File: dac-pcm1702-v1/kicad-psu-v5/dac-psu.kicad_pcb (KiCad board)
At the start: 2 copper layers, 123.2 x 81.3 mm, 81 parts, among them J1 AC, J10 LED, J11 GND, J12 +5V, J13 GND, J14 EARTH, J15 +17V, J16 -17V, J2 GND, J3 AC, J4 +15V, J5 GND, J6 -15V, J7 +5V, J8 GND, J9 -5V, U1 LM317_TO-220, U2 LT3045xMSE, U3 LT3094xMSE, U4 LT3045xMSE, U5 LT3094xMSE, U6 LM317_TO-220, U7 LM337_TO220

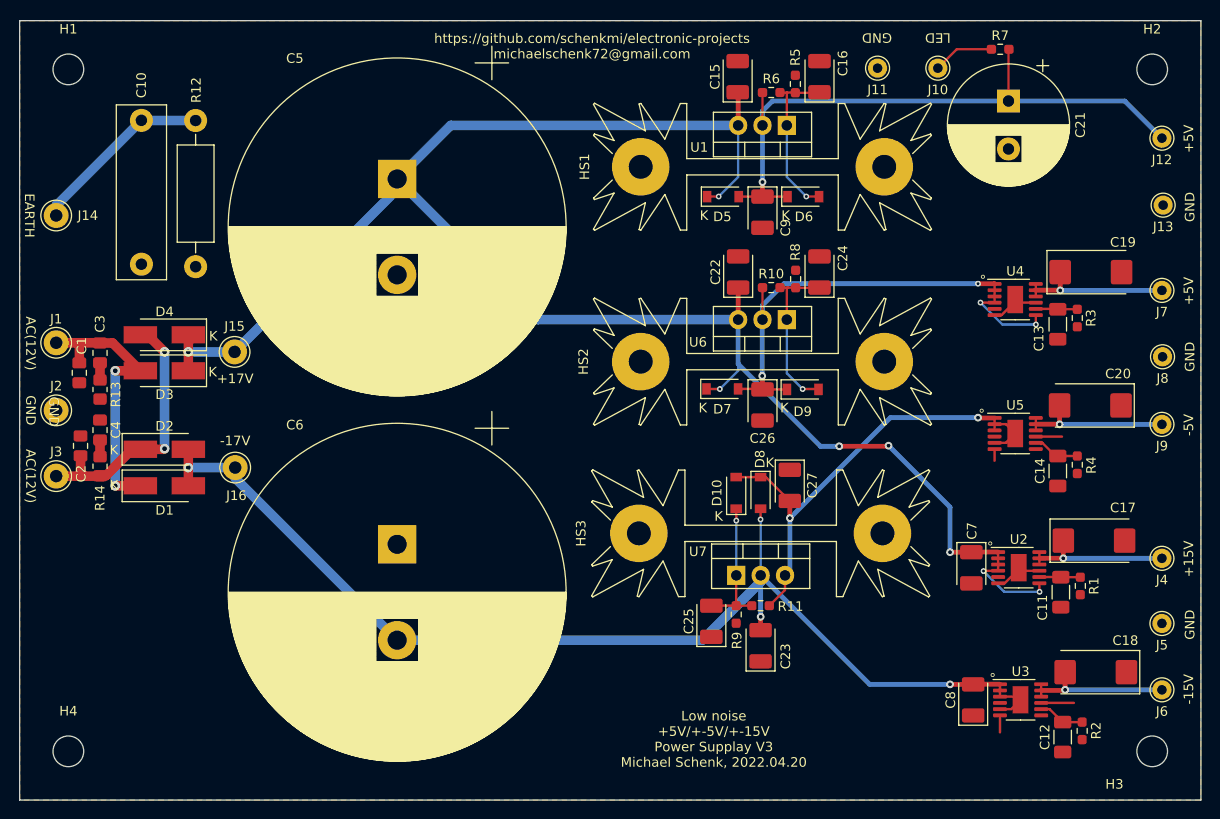
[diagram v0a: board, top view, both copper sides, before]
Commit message: Finalize V5 PSU
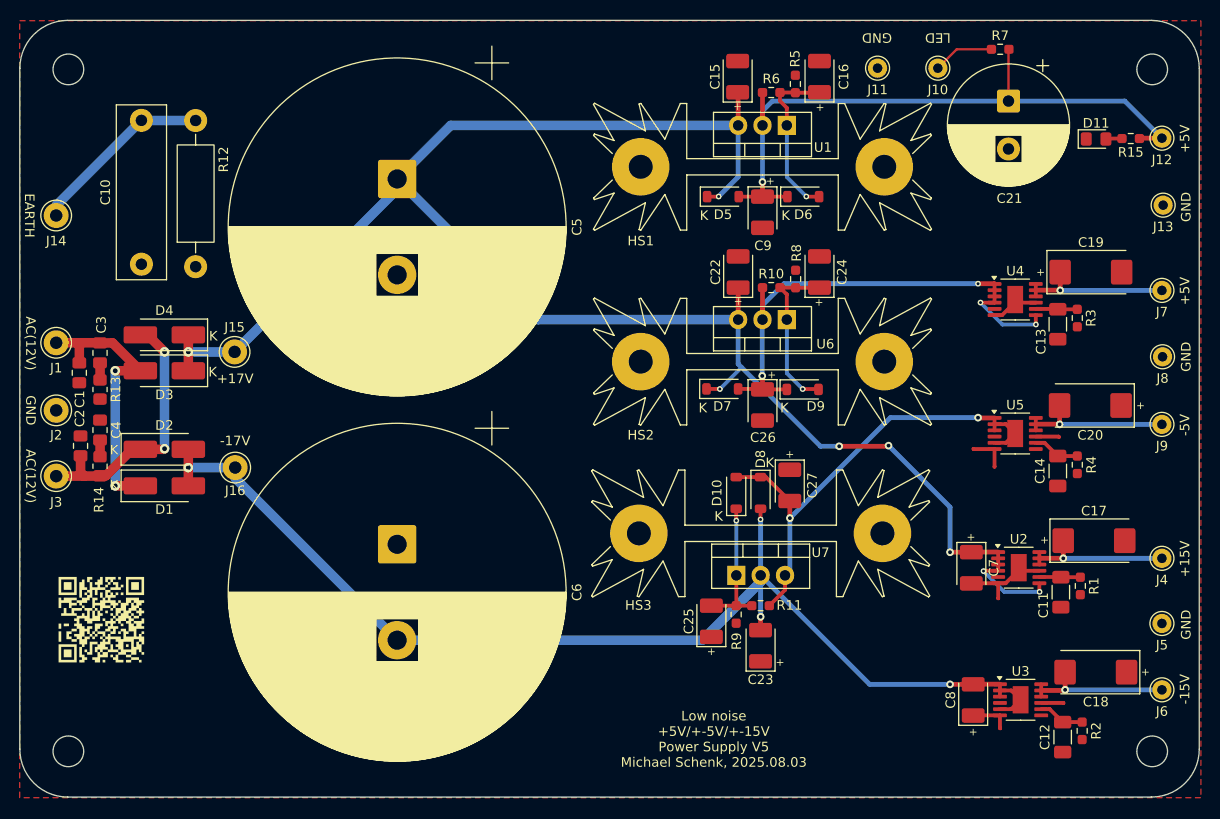
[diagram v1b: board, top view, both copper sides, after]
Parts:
- added D11: LED, LED_SMD:LED_0805_2012Metric_Pad1.15x1.40mm_HandSolder, F.Cu at (206.2, 61.9)
- added G***: LOGO, LOGO, F.Cu at (102.5, 112.0)
- added R15: 330R, Resistor_SMD:R_0603_1608Metric_Pad0.98x0.95mm_HandSolder, F.Cu at (209.9, 61.8)
- C15, C16, C22, C23, C24, C25, C26, C27, C7, C8, C9: footprint Capacitor_Tantalum_SMD:CP_EIA-3528-21_Kemet-B_Pad1.50x2.35mm_HandSolder -> Capacitor_Tantalum_SMD:CP_EIA-3528-21_Kemet-B_HandSolder
- C17, C18, C19, C20: value 47uF -> 47uF/25V; footprint Capacitor_Tantalum_SMD:CP_EIA-7343-31_Kemet-D_Pad2.25x2.55mm_HandSolder -> Capacitor_Tantalum_SMD:CP_EIA-7343-31_Kemet-D_HandSolder
- U2, U3, U4, U5: footprint Package_SO:MSOP-12-1EP_3x4mm_P0.65mm_EP1.65x2.85mm -> Package_SO:MSOP-12-1EP_3x4.039mm_P0.65mm_EP1.651x2.845mm
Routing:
- net GND: track 18.3 -> 28.0 mm
- net +17V: track 191.4 -> 186.7 mm
- net Net-(D5-A): track 66.5 -> 68.8 mm
- net Net-(D11-A): track 0.00 -> 1.70 mm
- net -17V: track 122.8 -> 123.5 mm
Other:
- board size 123.2 x 81.3 mm -> 123 x 81 mm
- board text added: "+"
- board text added: "Low noise +5V/+-5V/+-15V Power Supply V5 Michael Schenk, 2025.08.03"
- board text removed: "Low noise +5V/+-5V/+-15V Power Supplay V3 Michael Schenk, 2022.04.20"
- board text removed: "https://github.com/schenkmi/electronic-projects michaelschenk72@gmail.com"
- board text removed: "°"
